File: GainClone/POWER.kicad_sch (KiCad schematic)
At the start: 31 parts, among them J13 AC, J14 GND, J15 AC, J16 GND, J17 GND, J18 GND, Q6 MJD31CJ, Q7 MJD32CJ, U8 TPS7A39*

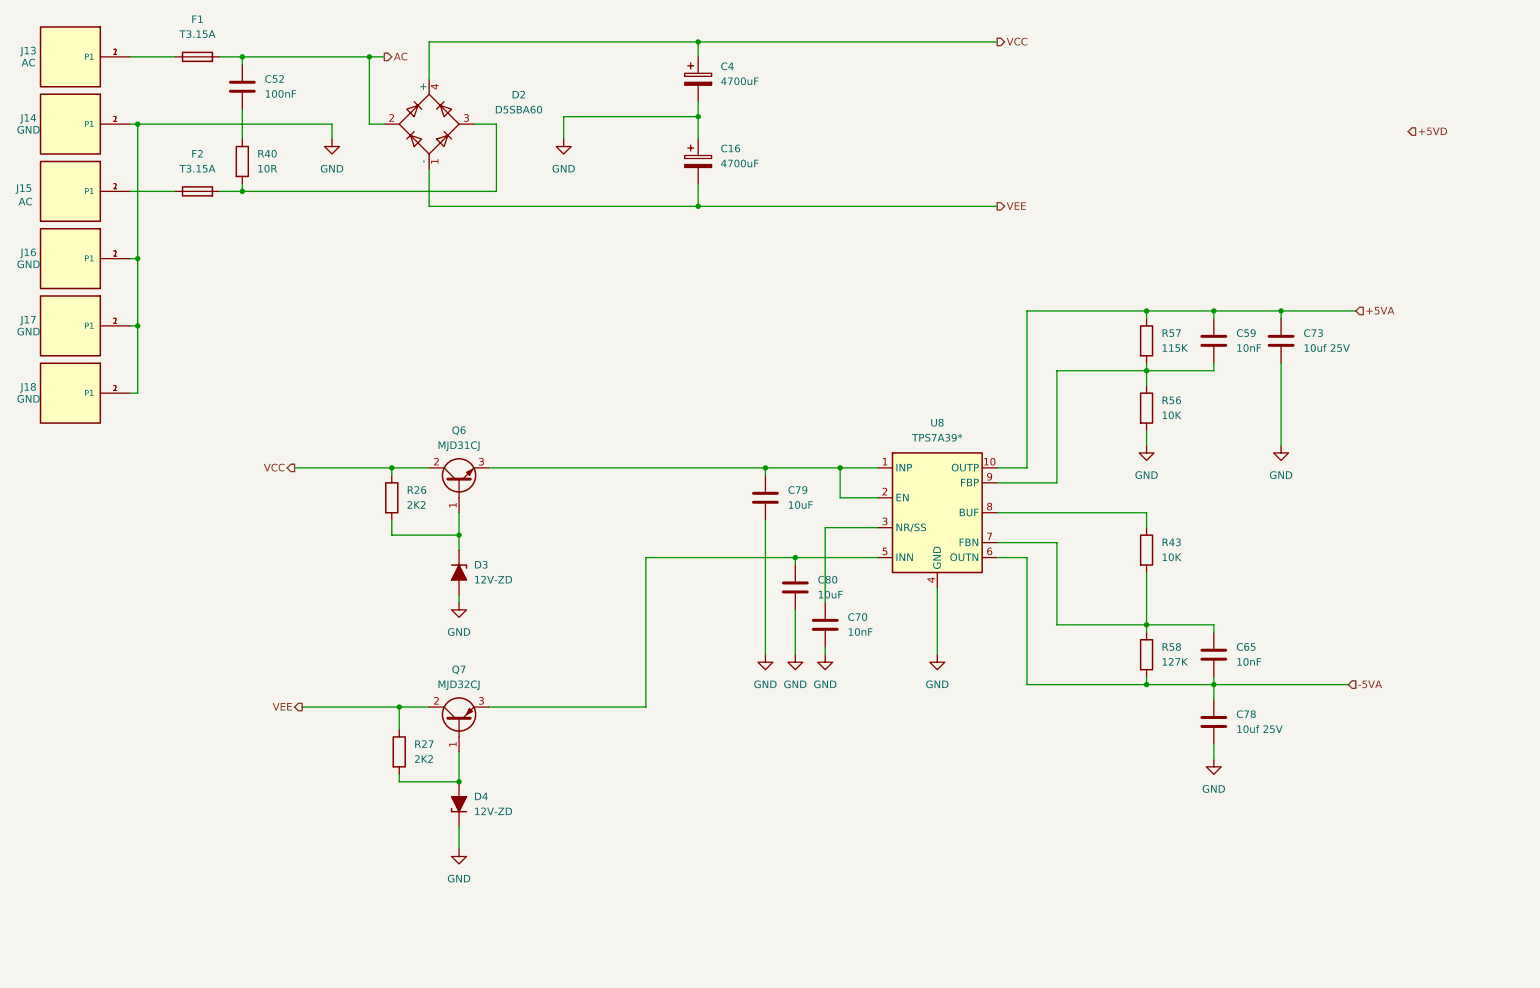
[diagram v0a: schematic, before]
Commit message: commit
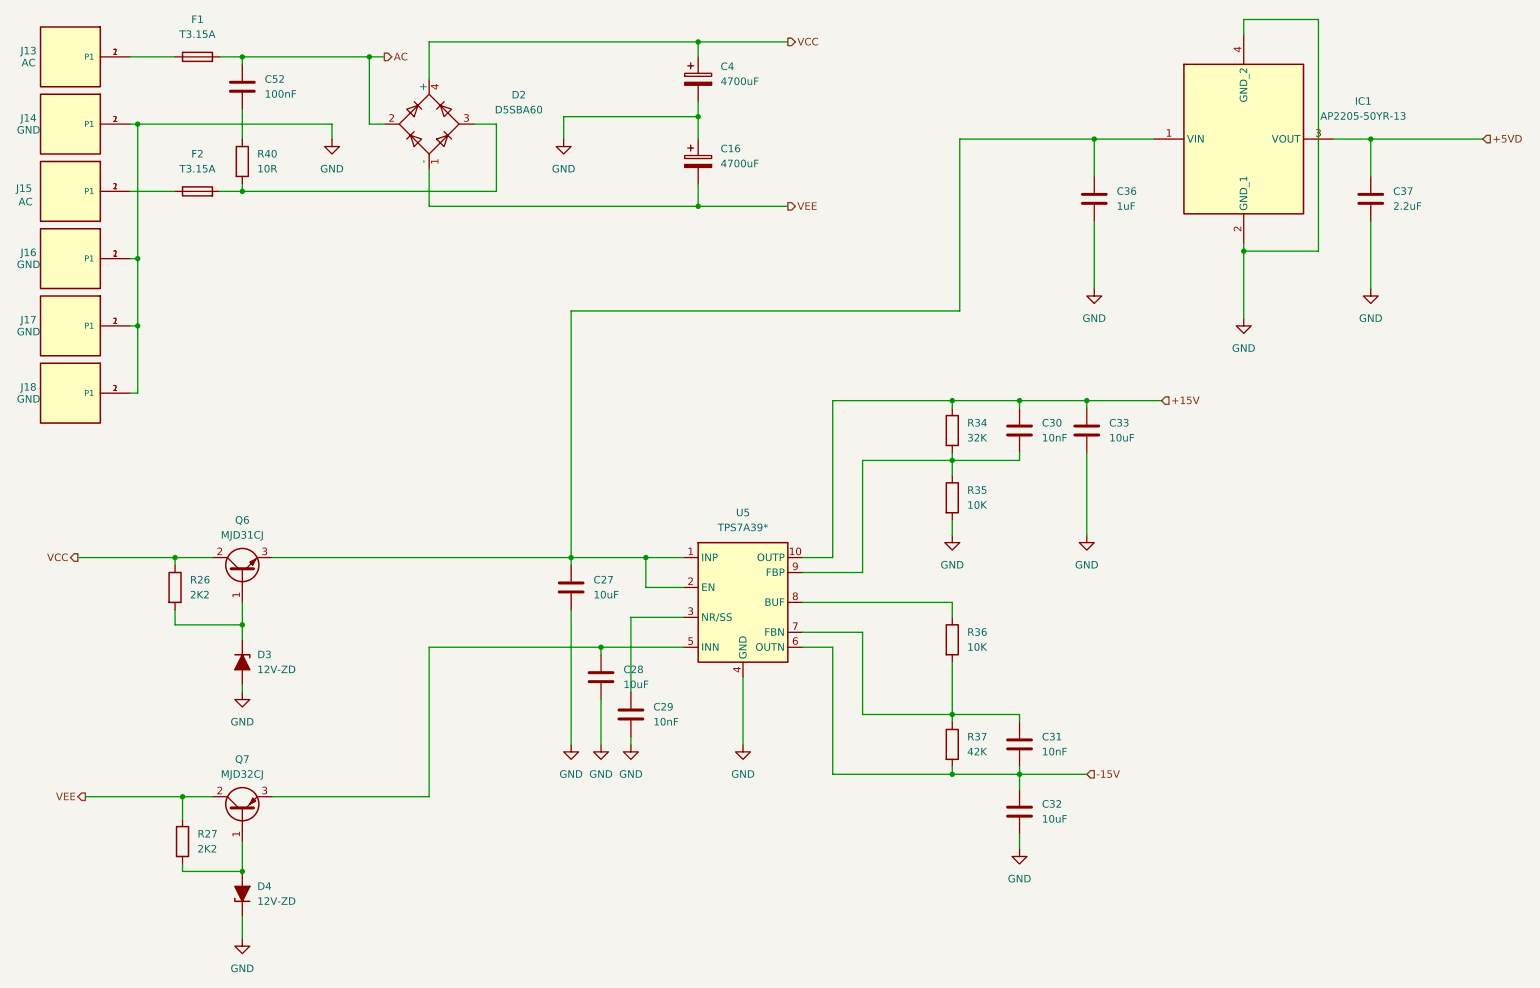
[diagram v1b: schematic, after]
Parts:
- removed C59, C65, C70: 10nF, Capacitor_SMD:C_0805_2012Metric_Pad1.18x1.45mm_HandSolder, symbol Device:C
- removed C73, C78: 10uf 25V, Capacitor_SMD:C_1206_3216Metric_Pad1.33x1.80mm_HandSolder, symbol Device:C
- removed C79, C80: 10uF, Capacitor_SMD:C_1206_3216Metric_Pad1.33x1.80mm_HandSolder, symbol Device:C
- removed R43, R56: 10K, Resistor_SMD:R_0805_2012Metric_Pad1.20x1.40mm_HandSolder, symbol Device:R
- removed R57: 115K, Resistor_SMD:R_0805_2012Metric_Pad1.20x1.40mm_HandSolder, symbol Device:R
- removed R58: 127K, Resistor_SMD:R_0805_2012Metric_Pad1.20x1.40mm_HandSolder, symbol Device:R
- removed U8: TPS7A39*, Package_SON:Texas_S-PVSON-N10_ThermalVias, symbol Regulator_Linear:TPS7A39
- added C27, C28, C32, C33: 10uF, Capacitor_SMD:C_1206_3216Metric_Pad1.33x1.80mm_HandSolder, symbol Device:C
- added C29, C30, C31: 10nF, Capacitor_SMD:C_0805_2012Metric_Pad1.18x1.45mm_HandSolder, symbol Device:C
- added C36: 1uF, Capacitor_SMD:C_1206_3216Metric_Pad1.33x1.80mm_HandSolder, symbol Device:C
- added C37: 2.2uF, Capacitor_SMD:C_0805_2012Metric_Pad1.18x1.45mm_HandSolder, symbol Device:C
- added IC1: AP2205-50YR-13, Package_TO_SOT_SMD:SOT-89-3, symbol Custom:AP2205-50YR-13
- added R34: 32K, Resistor_SMD:R_0805_2012Metric_Pad1.20x1.40mm_HandSolder, symbol Device:R
- added R35, R36: 10K, Resistor_SMD:R_0805_2012Metric_Pad1.20x1.40mm_HandSolder, symbol Device:R
- added R37: 42K, Resistor_SMD:R_0805_2012Metric_Pad1.20x1.40mm_HandSolder, symbol Device:R
- added U5: TPS7A39*, Package_SON:Texas_S-PVSON-N10_ThermalVias, symbol Regulator_Linear:TPS7A39
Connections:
- net +5VD: now also C37.1, IC1.3 (VOUT)
- net GND: now also C27.2, C28.2, C29.2, C32.2, C33.2, C36.2, C37.2, IC1.2 (GND_1), IC1.4 (GND_2), R35.2, U5.11 (GND), U5.4 (GND)
- net at Q7.3 (E): now also C28.1, U5.5 (INN)
- net at Q6.3 (E): now also C27.1, C36.1, IC1.1 (VIN), U5.1 (INP), U5.2 (EN)
- new net: C31.1, R36.2, R37.1, U5.7 (FBN)
- new net: R36.1, U5.8 (BUF)
- new net: C30.2, R34.2, R35.1, U5.9 (FBP)
- new net: C29.1, U5.3 (NR/SS)
- new net +15V: C30.1, C33.1, R34.1, U5.10 (OUTP)
- new net -15V: C31.2, C32.1, R37.2, U5.6 (OUTN)
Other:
- moved on the sheet: D3, D4, Q6, Q7, R26, R27
